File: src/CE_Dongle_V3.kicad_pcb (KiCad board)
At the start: 4 copper layers, 74 x 74 mm, 226 parts, among them J1 USB_C_Receptacle_USB2.0_16P, J10 Conn_01x02, J2 Conn_01x02, J3 Conn_01x02, J4 Conn_Coaxial, J5 Conn_Coaxial, J6 Conn_01x02, J7 8P8C_LED_Shielded, J8 Conn_01x02, J9 SIM_NANO_Socket, K1 G6K-2F-Y-TR DC5, K2 G6K-2F-Y-TR DC5, Q1 AO3401A, Q11 SI2308A, Q12 SI2308A, Q13 SI2308A, Q14 SI2308A, Q15 SI2308A, Q16 SI2308A, Q17 SI2308A, Q18 SI2308A, Q2 AO3401A, Q7 BC817-40-7-F, Q8 BC817-40-7-F, SW1 KH-6X6X4.3H-STM, SW2 KH-6X6X7H-STM, U1 ESP32-C6, U10 TMUX1208RSVR, U14 TPS54302DDCR, U15 TXS0104ERGYR, U16 LE910R1, U17 WS2812, U18 WS2812, U19 TPS54302DDCR, U2 SP3485, U20 WS2812, U3 W25Q64JVSSIQ, U4 TPS54302DDCR, U5 PCF8574RGTR(UMW), U6 PCF8574RGTR(UMW), U7 TMUX1208RSVR, U8 TMUX1208RSVR, U9 TMUX1208RSVR, Y1 40MHz

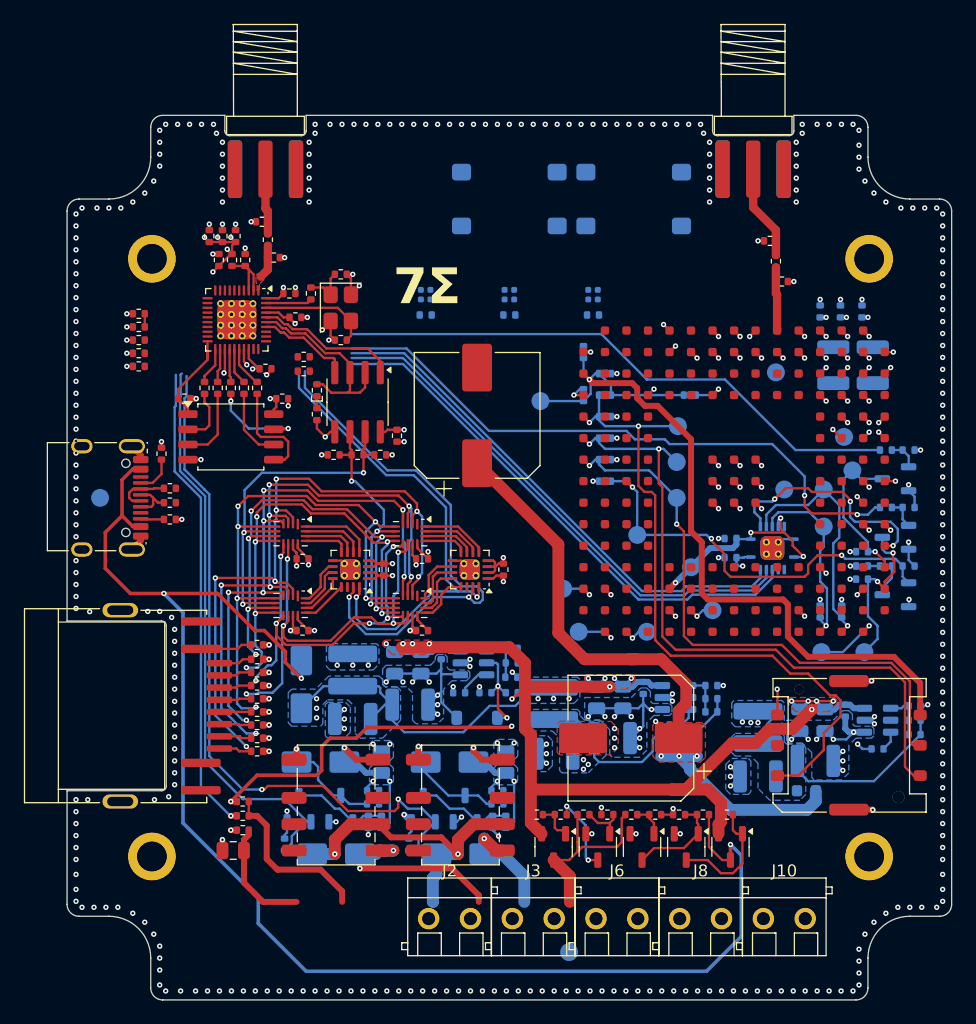
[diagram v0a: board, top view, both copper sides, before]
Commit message: floorplan changed, check in
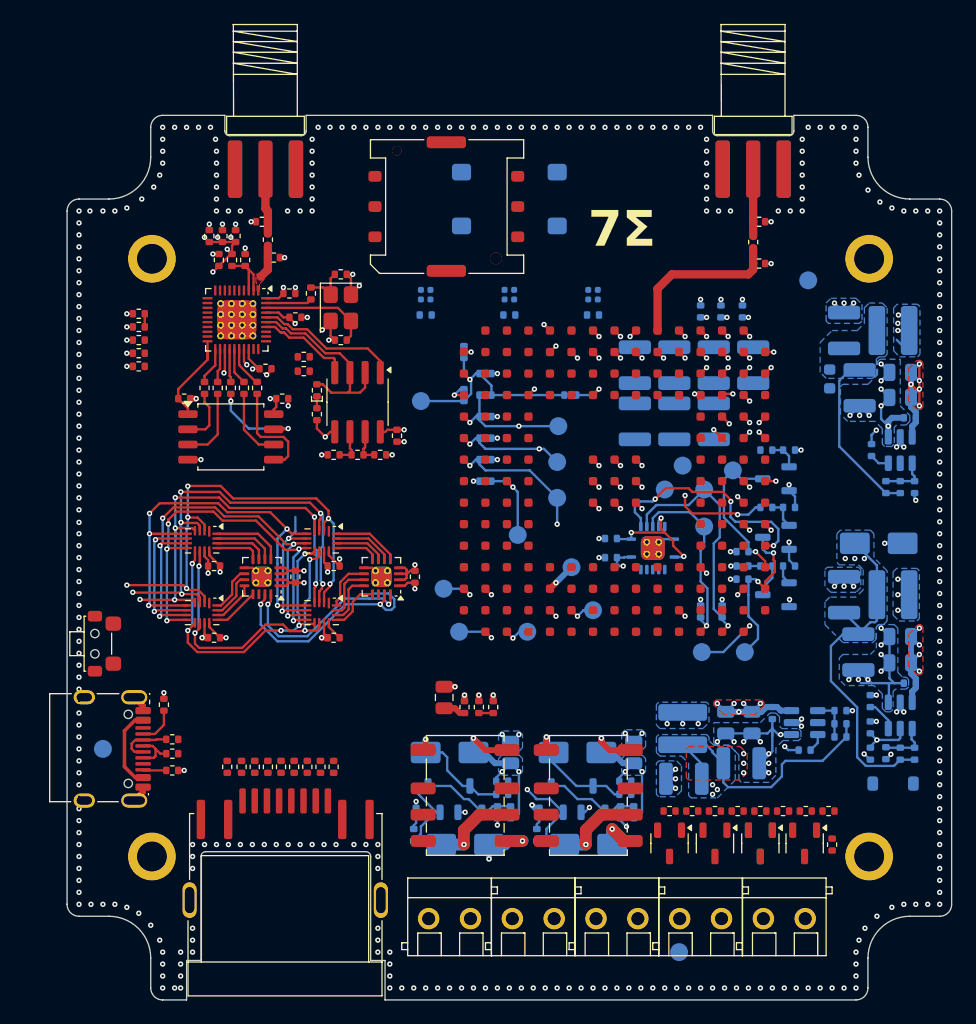
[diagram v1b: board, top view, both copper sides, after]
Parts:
- added C55: 47uF, 7Sigma:C_1210_3225Metric, B.Cu at (153.8, 88.6)
- added C56: 47uF, 7Sigma:C_1210_3225Metric, B.Cu at (157.1, 88.6)
- added C57: 47uF, 7Sigma:C_1210_3225Metric, B.Cu at (153.8, 83.9)
- C44, C45: value 470uF -> 47uF; footprint 7Sigma:CP_Elec_10x10 -> 7Sigma:C_1210_3225Metric; moved to B.Cu
- Q11: moved to B.Cu
- SW1: value KH-6X6X4.3H-STM -> TS24CA; footprint 7Sigma:SW-SMD_4P-L6.0-W6.0-P4.50-LS9.0-H4.3 -> 7Sigma:SW-SMD_TS24CA; moved to F.Cu
- moved SW1 57.8 mm to (106.1, 107.2), turned to 90 degrees
- moved J9 56.3 mm to (134.7, 70.6)
- moved D11 49.7 mm to (170.9, 98.8), turned to 0 degrees
- moved L6 45.6 mm to (172.1, 103.1), turned to 180 degrees
- moved C93 42.4 mm to (168.0, 103.1), turned to 90 degrees
- moved C87 42.4 mm to (172.7, 106.6), turned to 180 degrees
- moved C21 40.1 mm to (172.7, 108.8), turned to 180 degrees
- moved C92 39.3 mm to (173.5, 110.5), turned to 180 degrees
- moved C42 38.0 mm to (168.0, 81.0), turned to 90 degrees
- moved C83 37.8 mm to (169.2, 107.9), turned to -90 degrees
- moved U19 36.0 mm to (172.7, 113.2), turned to -90 degrees
- moved D12 35.2 mm to (172.1, 118.9), turned to 0 degrees
- moved L5 35.1 mm to (172.1, 81.0), turned to 180 degrees
- moved C82 34.8 mm to (173.9, 116.4), turned to 90 degrees
- moved FB1 34.5 mm to (166.8, 85.0), turned to -90 degrees
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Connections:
- SW1 pad 2: GND -> /MCU/RST
- SW1 pad 3: /MCU/RST -> (no net)
- SW1 pad 4: /MCU/RST -> (no net)
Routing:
- net GND: track 627.2 -> 405.9 mm, vias 458 -> 462
- net /PWR/VBUS: track 122.6 -> 8.37 mm, vias 3 -> 1
- net 3V3: track 194.6 -> 106.2 mm, vias 22 -> 19
- net /PWR/VSUPPLY: track 109.2 -> 34.4 mm
- net 5V0: track 121.3 -> 67.2 mm, vias 13 -> 11
- net 3V8: track 72.4 -> 19.9 mm, vias 12 -> 9
- net /MISC/RY2_CTRL: track 59.0 -> 7.49 mm, vias 2 -> 1
- net /LTE/SIM_VCC: track 67.7 -> 17.7 mm
- net /LTE/PWR_CYCLE: track 48.2 -> 0.00 mm
- net /LTE/SIM_CLK: track 55.6 -> 9.28 mm
- net /LTE/SIM_DAT: track 56.6 -> 10.6 mm
- net /LTE/UART_TX: track 44.8 -> 0.00 mm
- net /LTE/UART_RX: track 44.2 -> 0.00 mm
- net /LTE/SHUTDOWN: track 51.7 -> 7.74 mm
- net /LTE/PWR_MON: track 43.6 -> 0.00 mm
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- removed copper zone on F.Cu, net 3V8
- removed copper zone on In2.Cu, net GND
- removed copper zone on In2.Cu, net Net-(U19-SW)
- removed copper zone on In2.Cu, net Net-(U4-SW)
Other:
- outline, holes or cut-outs redrawn
